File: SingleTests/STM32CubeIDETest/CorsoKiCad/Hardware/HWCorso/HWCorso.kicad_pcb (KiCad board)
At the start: 4 copper layers, 80 x 80 mm, 48 parts, among them J1 USB_B_Mini, J2 BATTERY, J3 I2C_CONN, J4 SWD_CONN, J5 USART6_CONN, Q1 AO3401A, SW1 SW_SPDT, U1 STM32F401RCT6, U2 MP2359DJ-LF-Z, U3 USBLC6-2SC6, Y1 16MHz

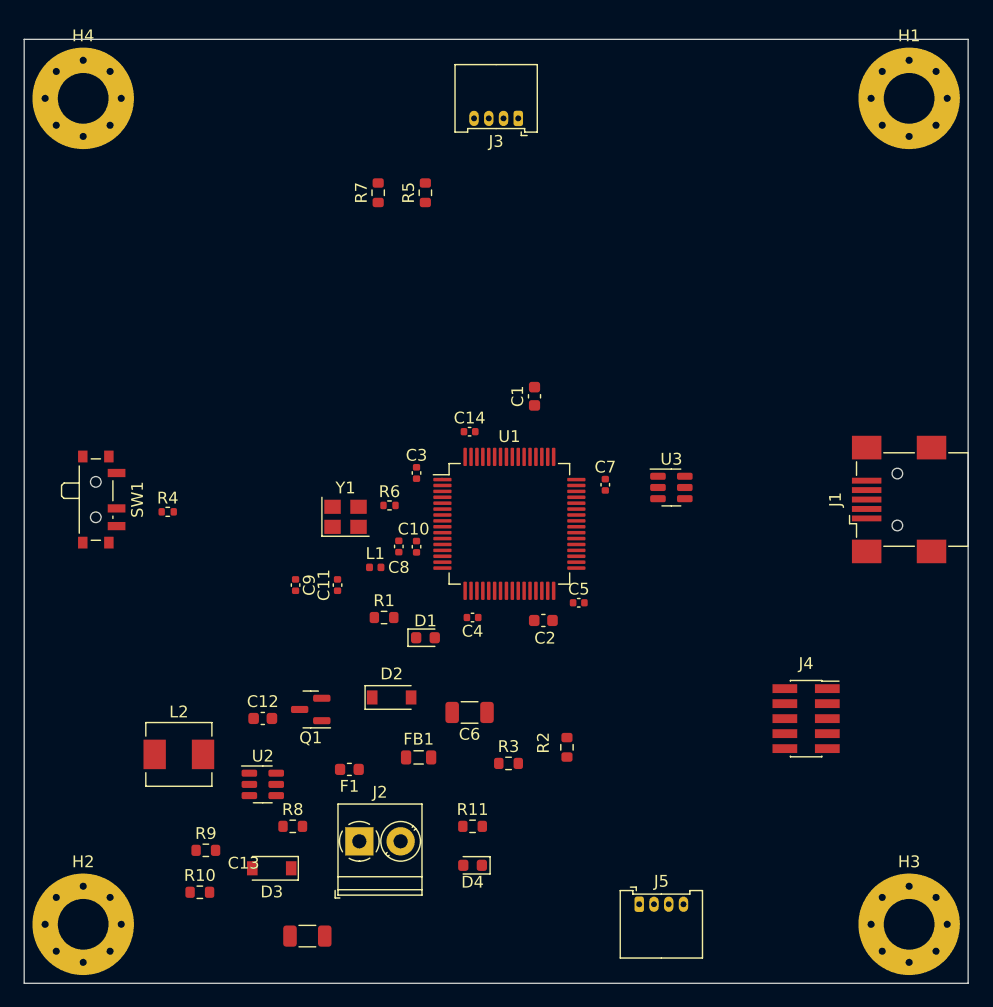
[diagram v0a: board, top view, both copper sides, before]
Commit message: Layout della scheda
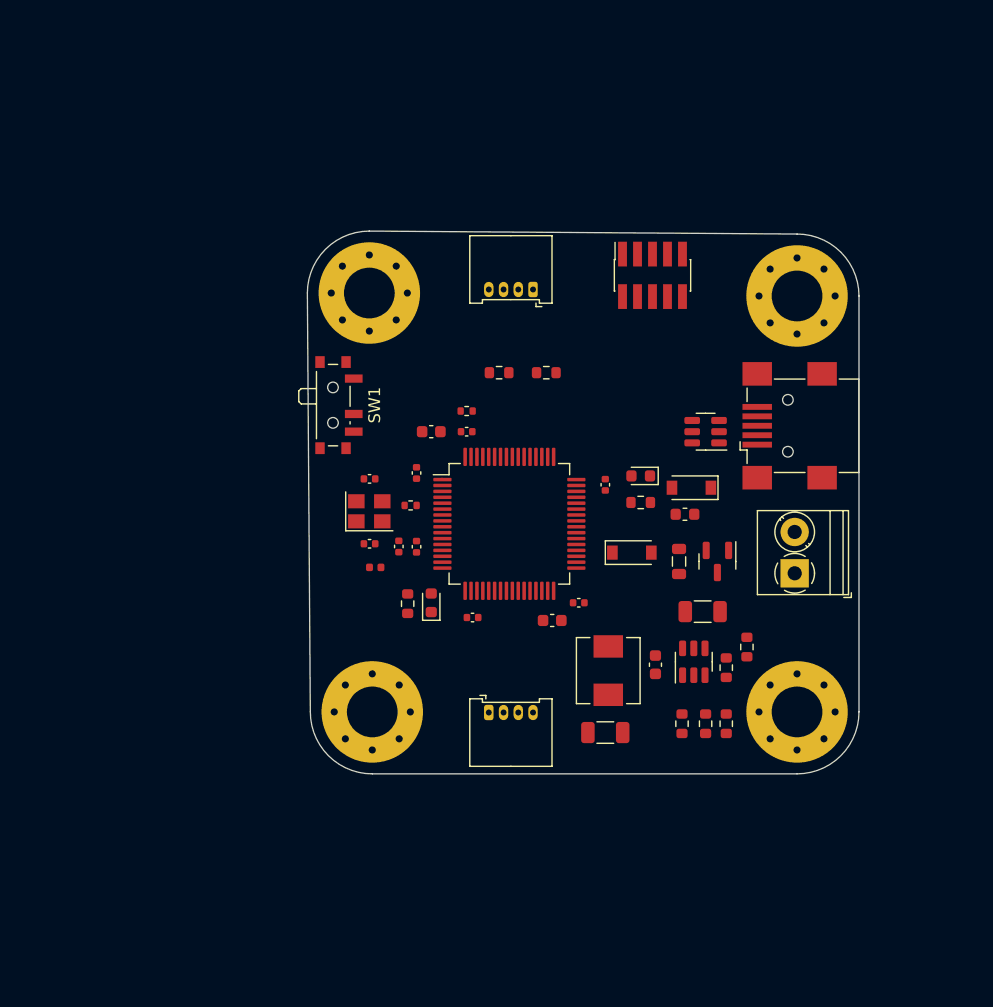
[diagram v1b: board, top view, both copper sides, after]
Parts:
- moved R10 46.8 mm to (89.5, 116.0), turned to -90 degrees
- moved R9 43.7 mm to (87.8, 116.0), turned to 90 degrees
- moved J2 43.3 mm to (95.3, 103.2), turned to 90 degrees
- moved D3 40.6 mm to (81.5, 101.5), turned to 0 degrees
- moved J4 39.8 mm to (83.2, 78.0), turned to 90 degrees
- moved U2 38.0 mm to (86.8, 110.8), turned to 90 degrees
- moved L2 37.1 mm to (79.5, 111.5), turned to -90 degrees
- moved Q1 36.7 mm to (88.8, 102.2), turned to -90 degrees
- moved D4 35.9 mm to (82.2, 95.0)
- moved F1 35.7 mm to (86.0, 98.2)
- moved R8 34.1 mm to (85.8, 116.0), turned to -90 degrees
- moved C12 33.6 mm to (83.5, 111.0), turned to 90 degrees
- moved D2 31.0 mm to (86.5, 96.0), turned to 180 degrees
- moved R11 30.9 mm to (82.2, 97.2)
- moved C13 30.6 mm to (79.2, 116.8), turned to 180 degrees
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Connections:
- F1 pad 1: +12V -> Net-(D2-Pad1)
- F1 pad 2: Net-(Q1-Pad3) -> Net-(F1-Pad2)
- FB1 pad 1: Net-(D2-Pad1) -> Net-(F1-Pad2)
- Q1 pad 3: Net-(Q1-Pad3) -> +12V
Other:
- board size 80 x 80 mm -> 46.8 x 46 mm

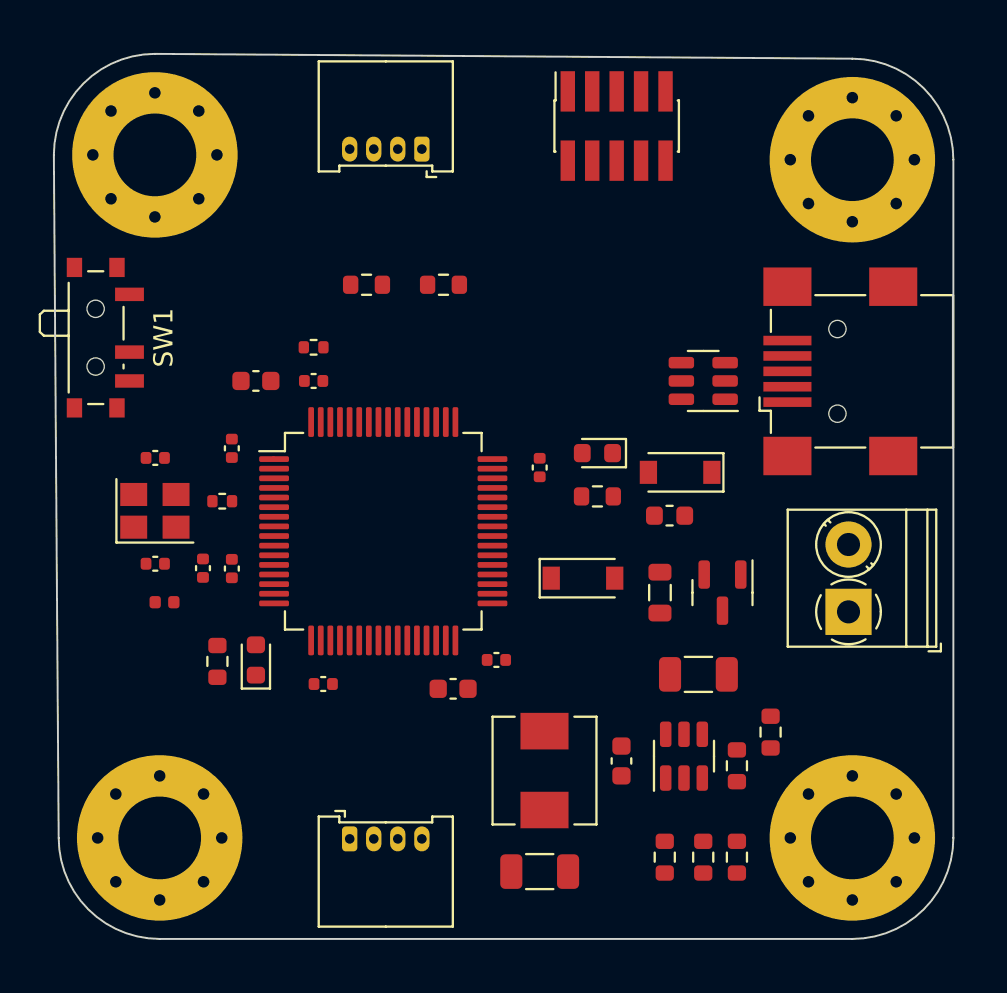
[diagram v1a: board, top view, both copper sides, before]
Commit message: Routing della scheda
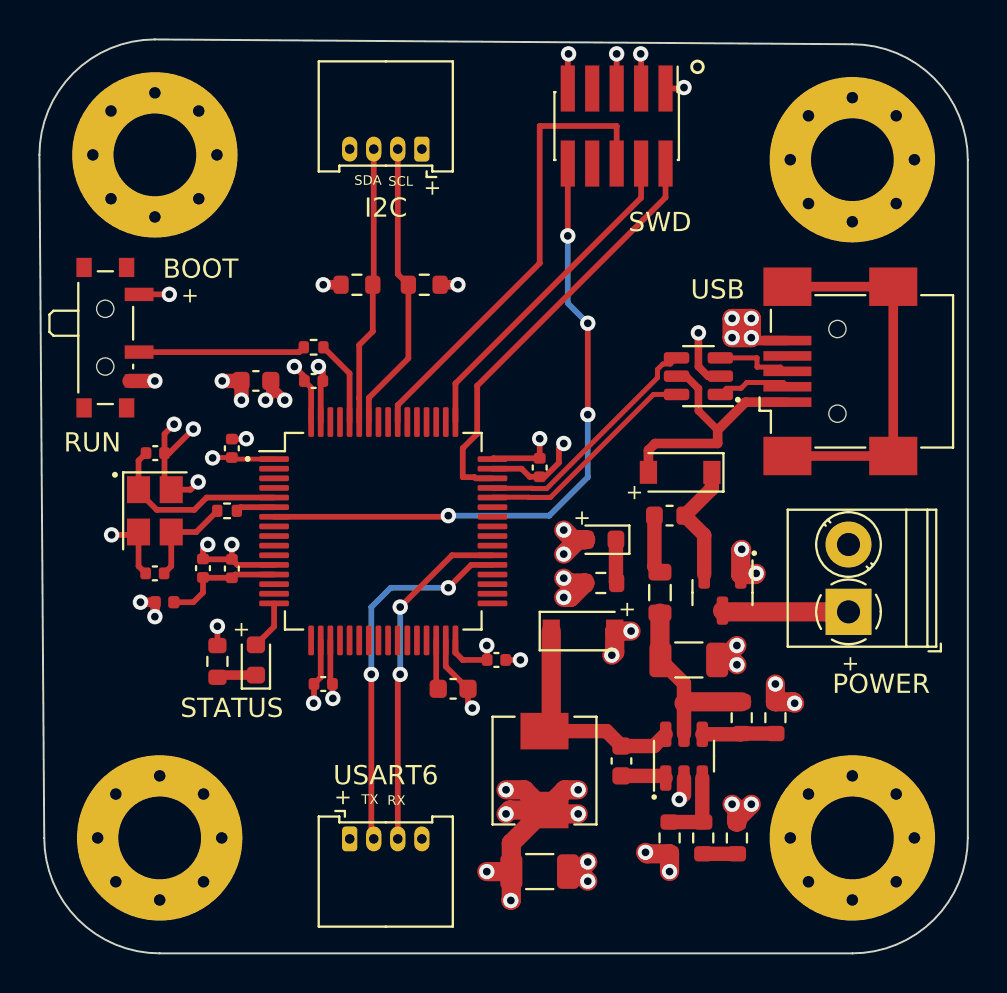
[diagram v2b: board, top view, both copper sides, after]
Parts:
- J4: footprint Connector_PinSocket_1.27mm:PinSocket_2x05_P1.27mm_Vertical_SMD -> Connector_PinHeader_1.27mm:PinHeader_2x05_P1.27mm_Vertical_SMD
- moved C11 6.00 mm to (59.2, 101.2)
- moved C9 5.75 mm to (59.3, 95.0)
- moved D4 4.50 mm to (82.4, 99.5)
- moved R11 4.50 mm to (82.4, 101.8)
- moved D3 2.75 mm to (81.5, 104.2)
- moved R2 2.51 mm to (89.8, 108.8)
- moved R8 1.03 mm to (86.0, 115.0)
- moved R10 1.00 mm to (89.5, 115.0)
- moved R5 1.00 mm to (73.2, 86.2)
- moved R9 1.00 mm to (87.8, 115.0)
- moved C6 0.90 mm to (87.0, 105.8)
- moved R3 0.79 mm to (91.5, 108.8)
- moved R6 0.56 mm to (63.0, 98.0)
- moved R7 0.50 mm to (69.8, 86.2)
- moved SW1 0.50 mm to (57.0, 89.0)
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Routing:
- net GND: track 0.00 -> 69.2 mm, vias 0 -> 39
- net BUCK_VOUT_3V3: track 0.05 -> 44.8 mm, vias 0 -> 23
- net NRST: track 0.00 -> 33.9 mm, vias 0 -> 4
- net SWO: track 0.00 -> 24.2 mm
- net SWDIO: track 0.00 -> 22.2 mm
- net unconnected-(J1-Pad6): track 0.00 -> 19.8 mm
- net USART6_TX: track 0.00 -> 19.3 mm, vias 0 -> 2
- net USART6_RX: track 0.00 -> 18.0 mm, vias 0 -> 2
- net SWCLK: track 0.00 -> 17.4 mm
- net I2C1_SCL: track 0.00 -> 15.3 mm
- net I2C1_SDA: track 0.00 -> 14.5 mm
- net +5V: track 0.00 -> 13.8 mm
- net USB_D+: track 0.00 -> 12.6 mm
- net BUCK_SW: track 0.00 -> 12.2 mm
- net USB_D-: track 0.00 -> 11.8 mm
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- added copper zone on In2.Cu, net BUCK_VOUT_3V3
- added copper zone on In1.Cu, net GND
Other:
- board size 46.8 x 46 mm -> 48.2 x 47.5 mm
- board text added: "+"
- board text added: "BOOT"
- board text added: "I2C"
- board text added: "POWER"
- board text added: "REV 1.0"
- board text added: "RUN"
- board text added: "RX"
- board text added: "SCL"
- board text added: "SDA"
- board text added: "STATUS"
- board text added: "SWD"
- board text added: "TX"
- board text added: "USART6"
- board text added: "USB"
- board text added: "https://github.com/GiovanniRaseraF"
